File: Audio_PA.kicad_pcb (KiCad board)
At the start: 2 copper layers, 133.5 x 90 mm, 71 parts, among them P1 Audio_In, P2 TP, P3 TP, P4 +45VDC, P5 Audio_Out, P6 -45VDC, Q1 BCM856DS, Q10 2N3904, Q11 2N3906, Q12 IRFP240, Q13 IRFP9240, Q2 BCM856DS, Q3 MJE340, Q4 MJE350, Q5 MJE350, Q6 MJE340, Q7 BD139, Q8 MJE340, Q9 MJE350

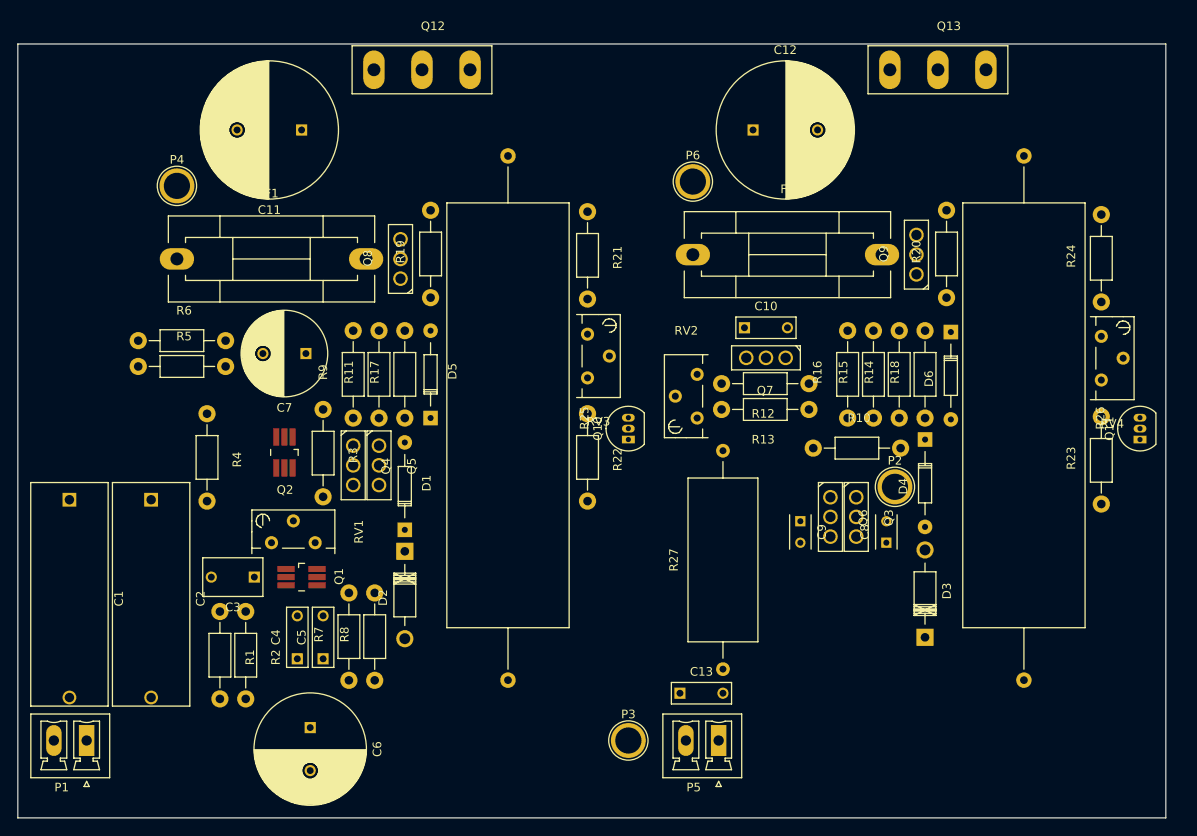
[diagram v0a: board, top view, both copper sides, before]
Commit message: Layout V1.1 + routing V1
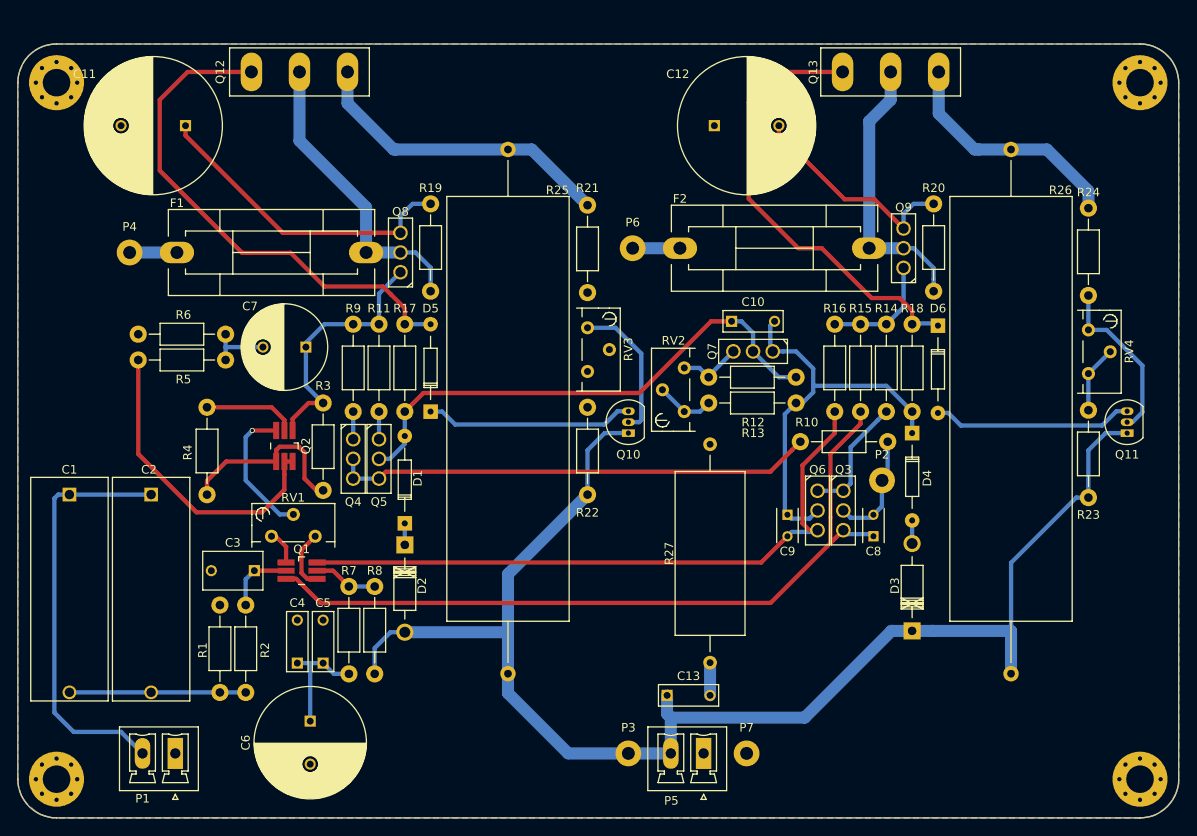
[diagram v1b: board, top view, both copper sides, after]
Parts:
- added P7: TP, Measurement_Points:Measurement_Point_Round-TH_Big, F.Cu at (158.8, 119.5)
- added REF**: MountingHole_3.2mm_M3_Pad_Via, Mounting_Holes:MountingHole_3.2mm_M3_Pad_Via, F.Cu at (204.5, 122.5)
- added REF**: MountingHole_3.2mm_M3_Pad_Via, Mounting_Holes:MountingHole_3.2mm_M3_Pad_Via, F.Cu at (78.5, 122.5)
- added REF**: MountingHole_3.2mm_M3_Pad_Via, Mounting_Holes:MountingHole_3.2mm_M3_Pad_Via, F.Cu at (78.5, 41.5)
- added REF**: MountingHole_3.2mm_M3_Pad_Via, Mounting_Holes:MountingHole_3.2mm_M3_Pad_Via, F.Cu at (204.5, 41.5)
- P2, P3, P4, P6: footprint Connectors:1pin -> Measurement_Points:Measurement_Point_Round-TH_Big
- moved Q12 14.3 mm to (106.8, 40.2)
- moved C11 13.5 mm to (93.5, 46.5)
- moved P6 10.4 mm to (145.5, 60.8)
- moved P1 10.4 mm to (92.3, 119.5)
- moved P4 9.50 mm to (87.0, 61.2)
- moved Q13 5.51 mm to (175.5, 40.2)
- moved C12 4.53 mm to (155.0, 46.5)
- moved P5 2.30 mm to (153.8, 119.5)
- moved C10 1.68 mm to (157.0, 69.2)
- moved C8 1.68 mm to (173.5, 94.2)
- moved C9 1.68 mm to (163.5, 91.8)
- moved D3 1.68 mm to (178.0, 105.2)
- moved D4 1.68 mm to (178.0, 82.2)
- moved D6 1.68 mm to (181.0, 69.8)
- moved F2 1.68 mm to (162.0, 60.8)
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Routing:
- net Net-(C13-Pad1): track 0.00 -> 166.2 mm
- net Net-(C8-Pad1): track 0.00 -> 90.0 mm
- net Net-(C9-Pad2): track 0.00 -> 76.4 mm
- net Net-(C10-Pad1): track 0.00 -> 61.3 mm
- net Net-(D5-Pad2): track 0.00 -> 60.2 mm
- net Net-(Q4-Pad2): track 0.00 -> 56.1 mm
- net Net-(D6-Pad1): track 0.00 -> 52.7 mm
- net Net-(C1-Pad1): track 0.00 -> 48.6 mm
- net Net-(C10-Pad2): track 0.00 -> 47.6 mm
- net Net-(Q12-Pad3): track 0.00 -> 37.5 mm
- net Net-(C11-Pad1): track 0.00 -> 36.9 mm
- net Net-(Q2-Pad5): track 0.00 -> 36.1 mm
- net Net-(F1-Pad2): track 0.00 -> 35.2 mm
- net Net-(F2-Pad2): track 0.00 -> 32.7 mm
- net Net-(C7-Pad1): track 0.00 -> 30.0 mm
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- added copper zone on B.Cu, net Earth
- added copper zone on F.Cu, net Earth
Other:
- board size 133.5 x 90 mm -> 135 x 90 mm
- net class Default: clearance 0.2 -> 0.25; trace_width 0.25 -> 0.5
- net class Power added: clearance 0.25, trace_width 1.4, via_dia 0.6, via_drill 0.4
- rule trace_clearance: 0.2 -> 0.25
